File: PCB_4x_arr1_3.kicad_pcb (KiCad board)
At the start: 4 copper layers, 50 x 76 mm, 0 parts

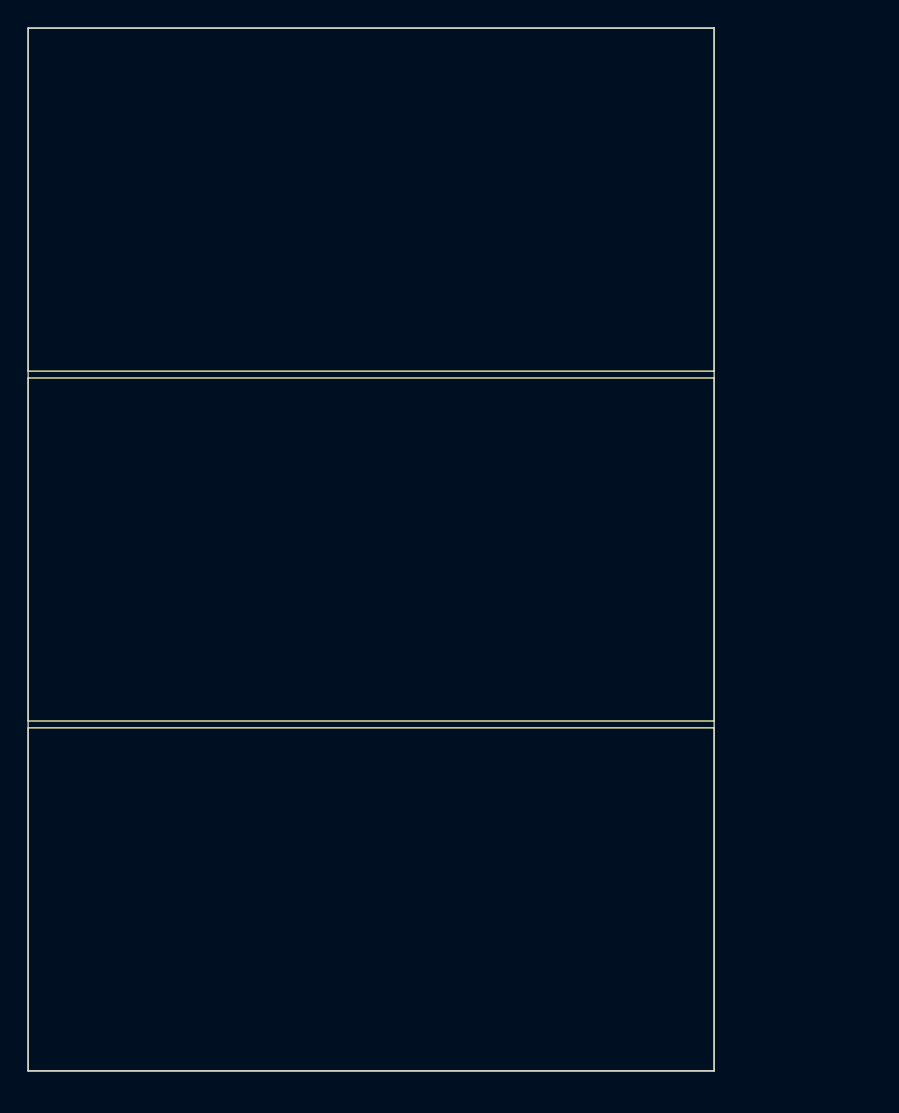
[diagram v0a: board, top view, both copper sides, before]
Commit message: Последние изменения в BOM
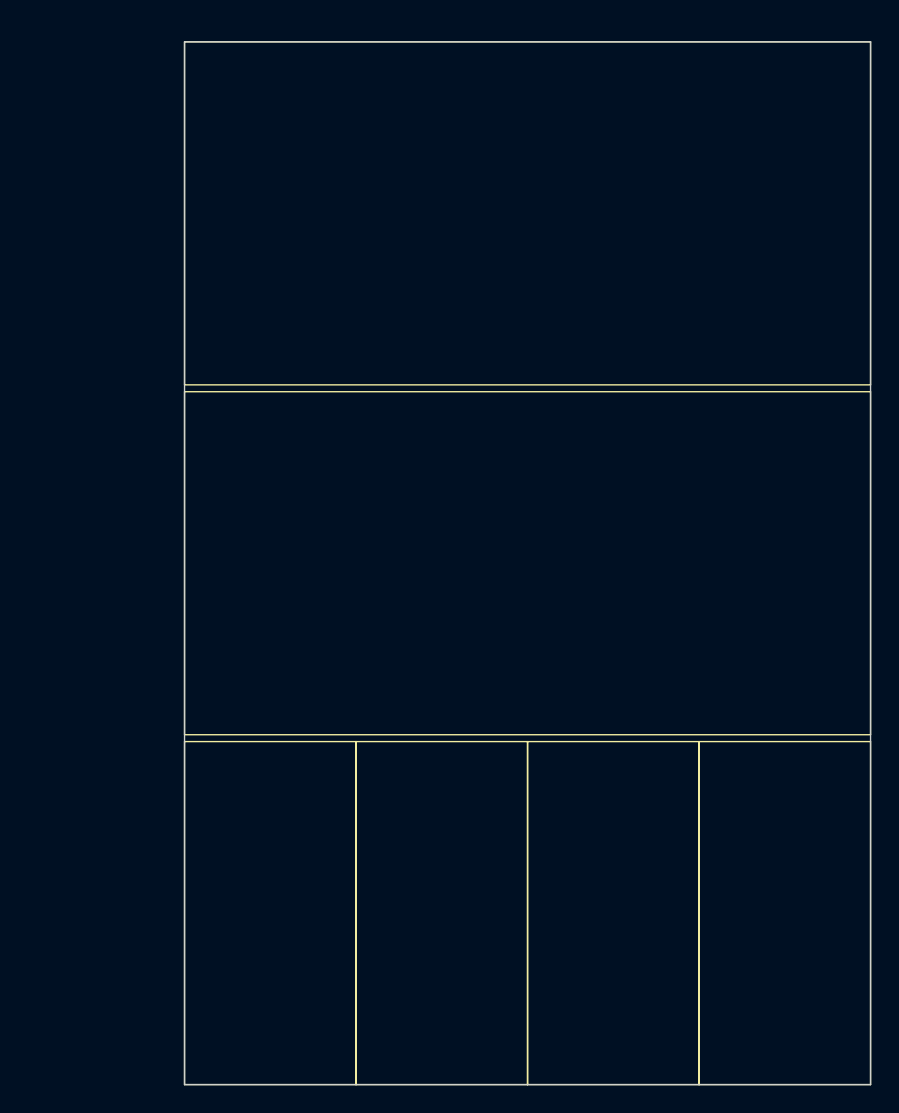
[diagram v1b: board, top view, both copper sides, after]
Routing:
- net /SCLq: track 0.00 -> 32.3 mm
- net /SCL: track 0.00 -> 22.9 mm
- net Net-(Q4-Pad2): track 0.00 -> 22.2 mm
- net /SDAq: track 0.00 -> 20.2 mm
- net Net-(Q7-Pad2): track 0.00 -> 19.4 mm
- net /SDA: track 0.00 -> 18.2 mm
- net Net-(Q8-Pad2): track 0.00 -> 15.3 mm
- net Net-(Q2-Pad2): track 0.00 -> 15.2 mm
- net Net-(Q6-Pad2): track 0.00 -> 14.5 mm
- net Net-(Q3-Pad2): track 0.00 -> 13.0 mm
- net Net-(Q1-Pad2): track 0.00 -> 5.09 mm
- net Net-(Q5-Pad2): track 0.00 -> 3.69 mm
